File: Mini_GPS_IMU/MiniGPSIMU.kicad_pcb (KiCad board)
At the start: 4 copper layers, 20 x 20 mm, 33 parts, among them U1 TCR2LE33LM, U2 STM32F072CBUx, U3 SAM-M8Q, U4 MPU-9250, U5 MS5611

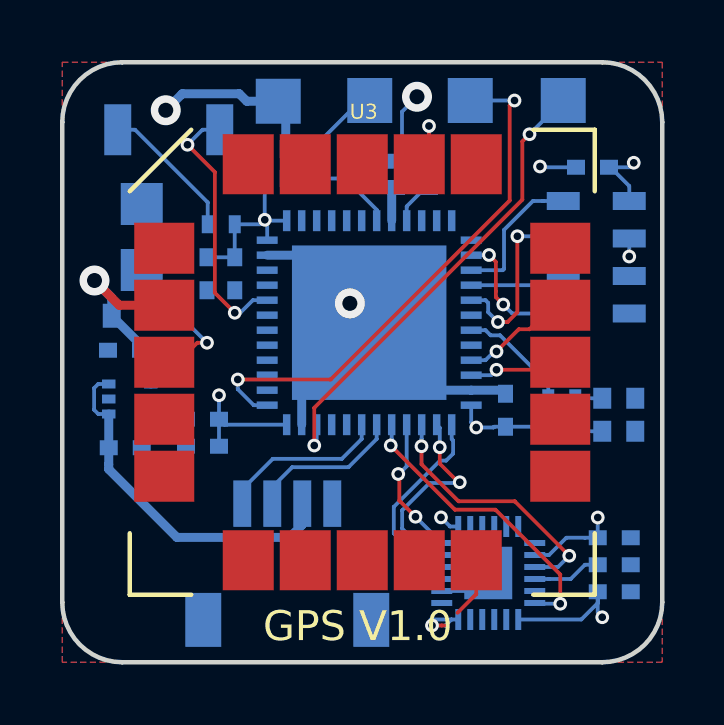
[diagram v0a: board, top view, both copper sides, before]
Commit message: Finished version 1.0 of GPS Diamond.
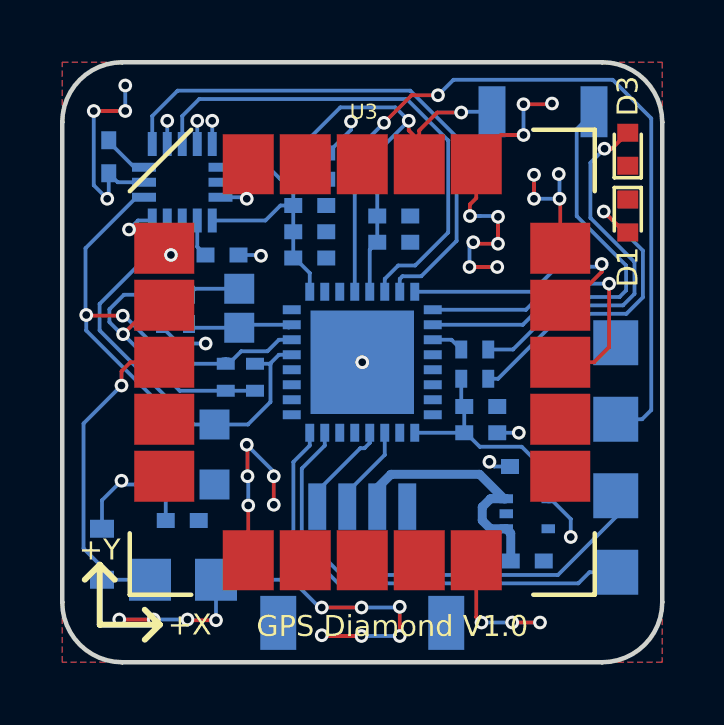
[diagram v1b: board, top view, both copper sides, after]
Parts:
- removed DFU: SW_Push, Buttons_Switches_SMD:SW_SPST_B3U-1000P
- removed GND, NRST, SWDCLK, SWDIO: TEST_1P, Measurement_Points:Measurement_Point_Square-SMD-Pad_Small
- removed Power, Status: LED, LEDs:LED_0402
- removed R2: 10k, Resistors_SMD:R_0402_NoSilk
- removed UART: CONN_01X04_MALE, Connectors_JST:JST_SH_SM04B-SRSS-TB_04x1.00mm_Angled
- added B1: SW_Push, jumper:SOLDER-JUMPER_1-WAY, B.Cu at (145.9, 98.2)
- added B2: SW_Push, Buttons_Switches_SMD:SW_SPST_B3U-3000P, B.Cu at (156.0, 91.7)
- added C14: 100nF, Capacitors_SMD:C_0402, B.Cu at (155.5, 103.5)
- added D1: LED, LEDs:LED_0402, F.Cu at (158.8, 95.1)
- added D3: LED, LEDs:LED_0402, F.Cu at (158.8, 92.9)
- added J1: CONN_01X04_MALE, Connectors_JST:JST_SH_SM04B-SRSS-TB_04x1.00mm_Angled, B.Cu at (150.0, 106.8)
- added J2: TEST_1P, Measurement_Points:Measurement_Point_Square-SMD-Pad_Small, B.Cu at (158.4, 101.9)
- added J3: TEST_1P, Measurement_Points:Measurement_Point_Square-SMD-Pad_Small, B.Cu at (158.4, 99.3)
- added J5: TEST_1P, Measurement_Points:Measurement_Point_Square-SMD-Pad_Small, B.Cu at (158.4, 104.5)
- added J6: TEST_1P, Measurement_Points:Measurement_Point_Square-SMD-Pad_Small, B.Cu at (158.4, 107.0)
- added R6: 10K, Resistors_SMD:R_0402, B.Cu at (146.4, 100.5)
- added R8: 10K, Resistors_SMD:R_0402, B.Cu at (145.4, 100.5)
- C1, C12: value 0.1uF -> 100nF; footprint Capacitors_SMD:C_0402_NoSilk -> Capacitors_SMD:C_0402
- C10, C8: value 10nF -> 100nF; footprint Capacitors_SMD:C_0402_NoSilk -> Capacitors_SMD:C_0402
- C11: value 0.1uF -> 100nF
- C13, C5, C6, C7: footprint Capacitors_SMD:C_0402_NoSilk -> Capacitors_SMD:C_0402
- C2: value 0.1uF -> 4.7uF; footprint Capacitors_SMD:C_0402_NoSilk -> Capacitors_SMD:C_0402
- C3: value 4.7uF -> 1uF; footprint Capacitors_SMD:C_0402_NoSilk -> Capacitors_SMD:C_0402
- C4: value 100nF -> 10nF; footprint Capacitors_SMD:C_0402_NoSilk -> Capacitors_SMD:C_0402
- C9: value 1uF -> 4.7uF; footprint Capacitors_SMD:C_0402_NoSilk -> Capacitors_SMD:C_0402
- R1, R3, R4, R7: footprint Resistors_SMD:R_0402_NoSilk -> Resistors_SMD:R_0402
- U2: value STM32F072CBUx -> STM32F042K6Ux; footprint Housings_DFN_QFN:QFN-48-1EP_7x7mm_Pitch0.5mm -> local:UFQFPN32
- U4: value MPU-9250 -> FXOS8700CQ; footprint MPU-9250:QFN40P300X300X105-25N -> local:FXOS8700CQ
- U5: value MS5611 -> MS5637; footprint local:MS5611 -> local:MS5637
- moved C12 17.2 mm to (145.3, 96.4)
- moved U4 16.5 mm to (144.0, 94.0), turned to 90 degrees
- moved U5 15.2 mm to (144.1, 103.1), turned to 0 degrees
- moved C10 15.0 mm to (148.2, 94.8)
- moved C11 14.5 mm to (144.0, 105.3)
- moved U1 13.8 mm to (155.5, 105.0)
- moved BT1 11.5 mm to (144.0, 107.2), turned to 90 degrees
- moved C7 9.98 mm to (151.1, 95.1), turned to 0 degrees
- moved C1 9.72 mm to (141.6, 93.2), turned to 270 degrees
- moved C13 9.44 mm to (148.2, 93.0), turned to 0 degrees
- moved C6 8.69 mm to (151.1, 96.0), turned to 0 degrees
- moved C8 8.49 mm to (153.9, 102.3), turned to 0 degrees
- moved C9 8.49 mm to (153.9, 101.5), turned to 0 degrees
- moved C2 8.40 mm to (148.2, 93.9), turned to 0 degrees
- moved D2 8.04 mm to (141.3, 106.4), turned to 90 degrees
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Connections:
- C1 pad 1: +5V -> Net-(C1-Pad1)
- C11 pad 1: Net-(C11-Pad1) -> +3V3
- C12 pad 1: +3V3 -> Net-(C12-Pad1)
- C5 pad 1: +3V3 -> +5V
- R7 pad 1: Net-(R7-Pad1) -> Net-(B1-Pad2)
- U2 pad 11: Net-(U2-Pad11) -> LED
- U2 pad 12: Net-(U2-Pad12) -> (no net)
- U2 pad 13: Net-(U2-Pad13) -> (no net)
- U2 pad 14: SPI1_NSS -> (no net)
- U2 pad 15: SPI1_SCK -> (no net)
- U2 pad 16: SPI1_MISO -> (no net)
- U2 pad 17: SPI1_MOSI -> +3V3
- U2 pad 18: Net-(U2-Pad18) -> (no net)
- U2 pad 19: LED -> USART1_TX
- U2 pad 2: Net-(U2-Pad2) -> (no net)
- U2 pad 20: Net-(U2-Pad20) -> USART1_RX
- U2 pad 21: USART3_TX -> (no net)
- U2 pad 22: USART3_RX -> (no net)
- U2 pad 23: GND -> Net-(J5-Pad1)
- U2 pad 24: +3V3 -> Net-(J6-Pad1)
- U2 pad 25: SPI2_NSS -> (no net)
- U2 pad 26: SPI2_SCK -> (no net)
- U2 pad 27: SPI2_MISO -> (no net)
- U2 pad 28: SPI2_MOSI -> (no net)
- U2 pad 29: IMU_INT -> I2C1_SCL
- U2 pad 3: Net-(U2-Pad3) -> (no net)
- U2 pad 30: UART1_TX -> I2C1_SDA
- U2 pad 31: UART1_RX -> Net-(B1-Pad2)
- U2 pad 32: Net-(U2-Pad32) -> (no net)
- U2 pad 33: Net-(U2-Pad33) -> GND
- U2 pad 5: Net-(U2-Pad5) -> +3V3
- U2 pad 6: Net-(U2-Pad6) -> IMU_INT1
- U2 pad 7: Net-(NRST1-Pad1) -> IMU_INT2
- U2 pad 8: GND -> USART2_TX
- U2 pad 9: +3V3 -> USART2_RX
- U3 pad 12: Net-(U3-Pad12) -> (no net)
- U3 pad 13: USART3_RX -> USART2_RX
- U3 pad 14: USART3_TX -> USART2_TX
- U3 pad 18: Net-(U3-Pad18) -> (no net)
- U3 pad 19: Net-(U3-Pad19) -> (no net)
- U3 pad 7: Net-(U3-Pad7) -> (no net)
- U3 pad 8: Net-(U3-Pad8) -> (no net)
- U3 pad 9: Net-(U3-Pad9) -> (no net)
- U4 pad 10: Net-(C11-Pad1) -> GND
- U4 pad 11: Net-(U4-Pad11) -> IMU_INT1
- U4 pad 12: IMU_INT -> GND
- U4 pad 13: +3V3 -> GND
- U4 pad 14: (no net) -> +3V3
- U4 pad 16: (no net) -> GND
- U4 pad 2: (no net) -> Net-(C12-Pad1)
- U4 pad 3: (no net) -> GND
- U4 pad 4: (no net) -> I2C1_SCL
- U4 pad 5: (no net) -> GND
- U4 pad 6: (no net) -> I2C1_SDA
- U4 pad 7: Net-(U4-Pad7) -> GND
- U4 pad 8: +3V3 -> Net-(C1-Pad1)
- U4 pad 9: SPI2_MISO -> IMU_INT2
- U5 pad 2: GND -> I2C1_SDA
- U5 pad 3: GND -> I2C1_SCL
- U5 pad 4: Net-(U5-Pad4) -> GND
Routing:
- net GND: track 23.6 -> 58.0 mm, vias 6 -> 47
- net Net-(J2-Pad1): track 0.00 -> 27.9 mm, vias 0 -> 2
- net IMU_INT2: track 0.00 -> 18.4 mm
- net Net-(SWDCLK1-Pad1): track 17.9 -> 0.00 mm, vias 2 -> 0
- net I2C1_SDA: track 0.00 -> 17.8 mm, vias 0 -> 2
- net IMU_INT1: track 0.00 -> 16.9 mm
- net Net-(J5-Pad1): track 0.00 -> 16.3 mm
- net +3V3: track 35.5 -> 51.6 mm, vias 9 -> 5
- net Net-(SWDIO1-Pad1): track 15.7 -> 0.00 mm, vias 2 -> 0
- net Net-(J6-Pad1): track 0.00 -> 15.4 mm
- net I2C1_SCL: track 0.00 -> 14.8 mm
- net Net-(B2-Pad1): track 0.00 -> 14.2 mm
- net Net-(D3-Pad2): track 0.90 -> 12.3 mm, vias 0 -> 1
- net Net-(R7-Pad1): track 10.4 -> 0.00 mm, vias 2 -> 0
- net USART2_RX: track 0.00 -> 10.3 mm, vias 0 -> 1
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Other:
- board text added: "+X"
- board text added: "+Y"
- board text added: "GPS Diamond V1.0"
- board text added: "NRST"
- board text added: "SWDCLK"
- board text added: "SWDIO"
- board text removed: "GPS V1.0"
